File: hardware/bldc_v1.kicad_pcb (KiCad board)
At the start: 4 copper layers, 124.1 x 121.1 mm, 63 parts, among them J1 Conn_01x06, J2 1x2_ScrewTerminal_65A, J3 Screw_Terminal_01x05, J4 RJ45, J5 Screw_Terminal_01x03, M1 IPB044N15N5, M2 IPB044N15N5, M3 IPB044N15N5, M4 IPB044N15N5, M5 IPB044N15N5, M6 IPB044N15N5, M7 STM32F4-DISCOVERY, U1 AD8205, U2 AD8205

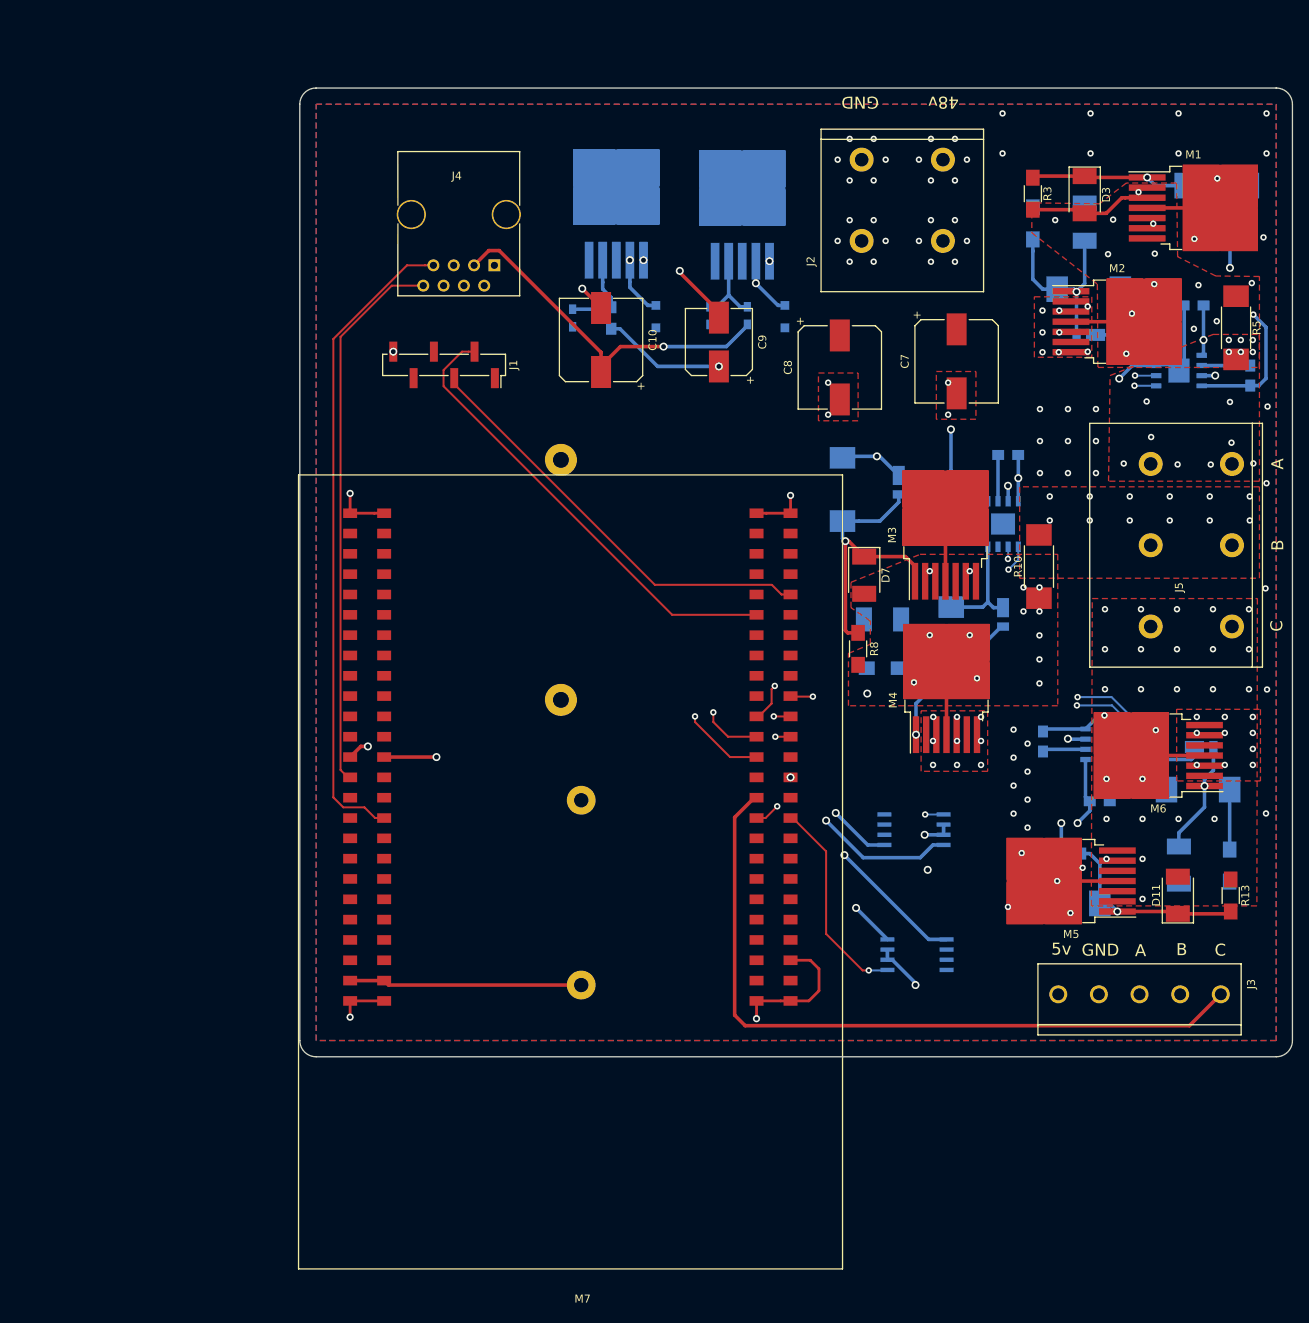
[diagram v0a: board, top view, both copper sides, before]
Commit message: updated routing and all plots
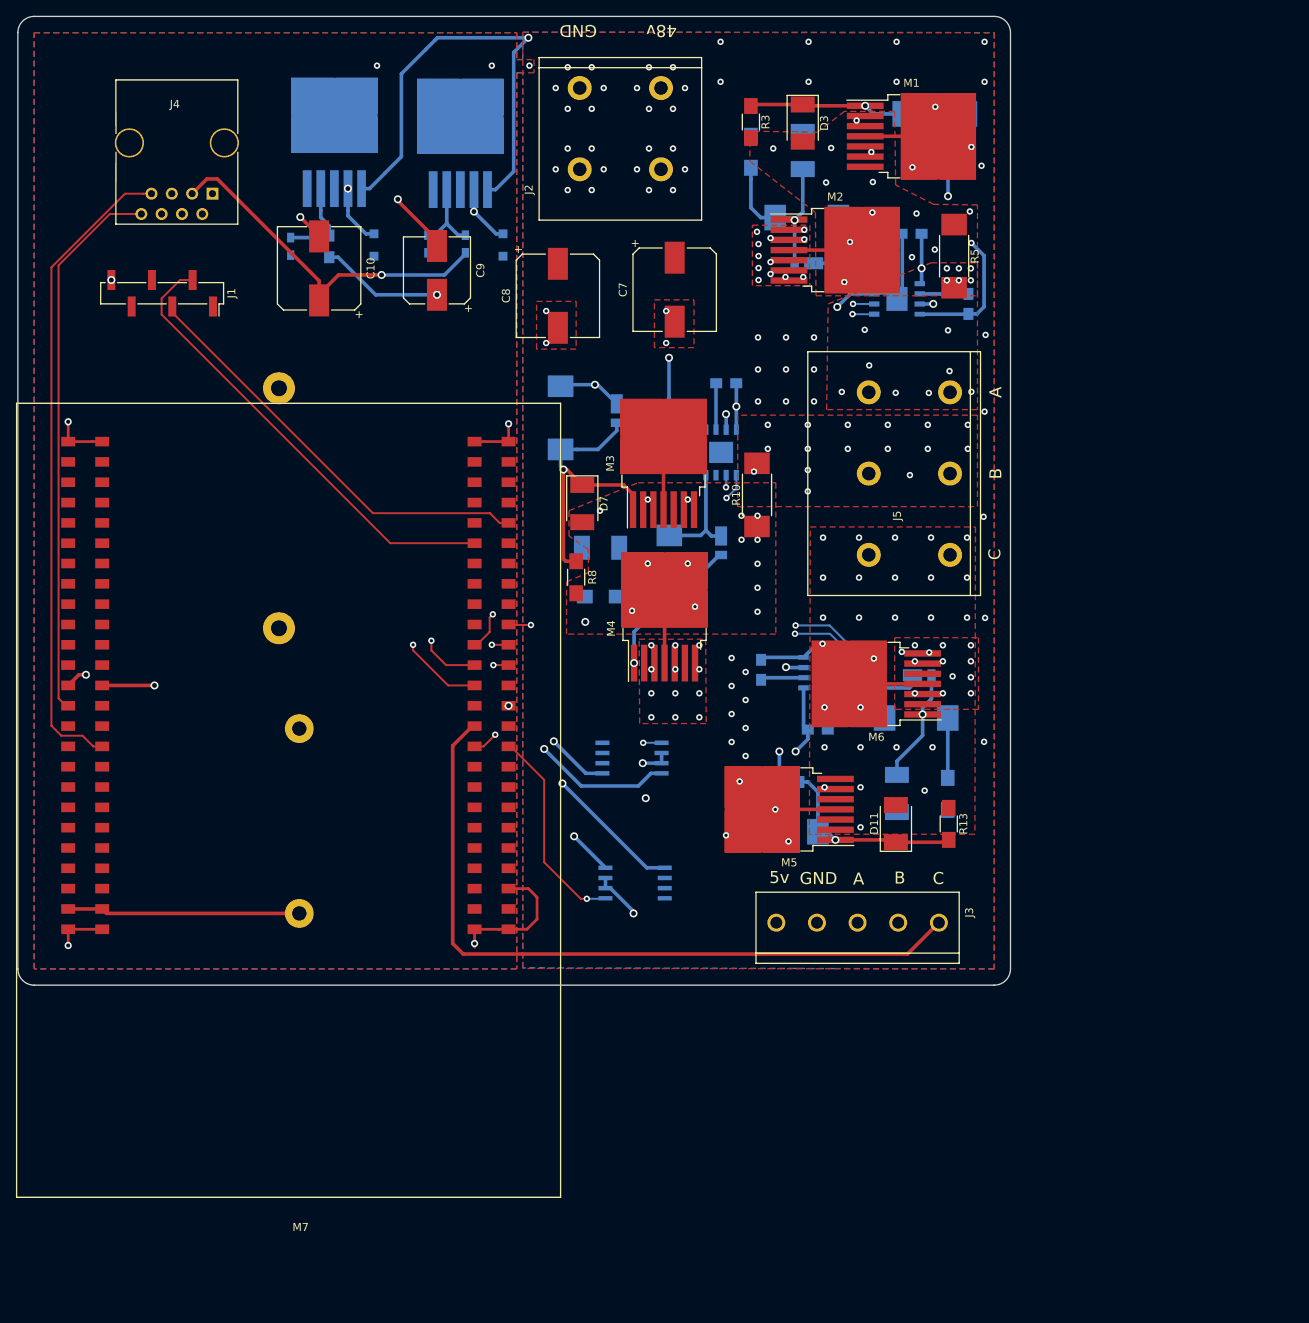
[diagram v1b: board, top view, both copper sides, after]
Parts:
- moved 12vConverter1 36.4 mm to (117.5, 38.8)
- moved 5vConverter1 36.4 mm to (133.3, 38.9)
- moved C1 36.4 mm to (166.5, 68.9)
- moved C10 36.4 mm to (115.6, 54.5)
- moved C2 36.4 mm to (170.9, 104.7)
- moved C3 36.4 mm to (196.8, 59.0)
- moved C4 36.4 mm to (189.7, 50.2)
- moved C5 36.4 mm to (158.8, 75.7)
- moved C6 36.4 mm to (178.0, 112.2)
- moved C7 36.4 mm to (160.1, 57.2)
- moved C8 36.4 mm to (145.5, 58.0)
- moved C9 36.4 mm to (130.4, 54.8)
- moved D1 36.4 mm to (192.8, 40.1)
- moved D10 36.4 mm to (190.7, 105.4)
- moved D11 36.4 mm to (187.7, 124.0)
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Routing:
- net /48v: track 27.4 -> 82.2 mm
- net /GND: track 63.0 -> 106.9 mm, vias 54 -> 66
- net /GateDriver/PhaseASource: track 145.9 -> 130.7 mm
- net /GateDriver/+12V: track 236.7 -> 237.8 mm
- net /MOSFETS/PhaseC: vias 26 -> 27
- net /MOSFETS/PhaseB: vias 13 -> 17
- net /GateDriver/PhaseBSource: vias 16 -> 17
